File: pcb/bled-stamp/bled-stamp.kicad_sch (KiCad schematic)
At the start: 38 parts, among them SW1 SW_Push, SW2 SW_Push, SW3 SW_Push, SW4 SW_Push, SW5 SW_Push, U1 RP2350A, U2 W25Q32RVXHJQ, X1 ABM8-272-T3

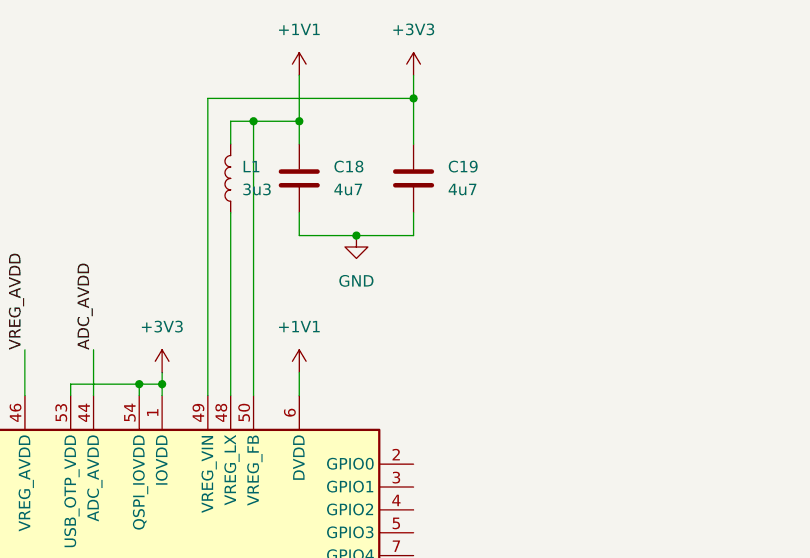
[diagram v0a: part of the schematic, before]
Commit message: wip
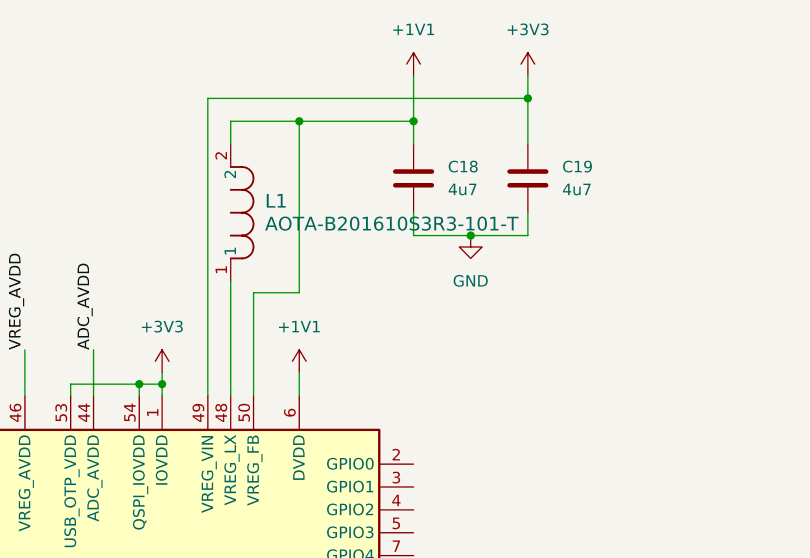
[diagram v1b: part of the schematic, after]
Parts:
- removed L1: 3u3, symbol Device:L
- added L1: AOTA-B201610S3R3-101-T, bled:IND_AOTA-B201610S_2p0x1p6x1p0_ABR-L, symbol bled:AOTA-B201610S3R3-101-T
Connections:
- net +1V1: now also L1.2
- net at U1.48 (VREG_LX): now also L1.1
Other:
- moved on the sheet: C18, C19
